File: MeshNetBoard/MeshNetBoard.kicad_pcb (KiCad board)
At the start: 2 copper layers, 35 x 21 mm, 9 parts, among them J1 Conn_01x02, U1 XIAO-ESP32-S3-DIP, U2 TPS631000DRLR

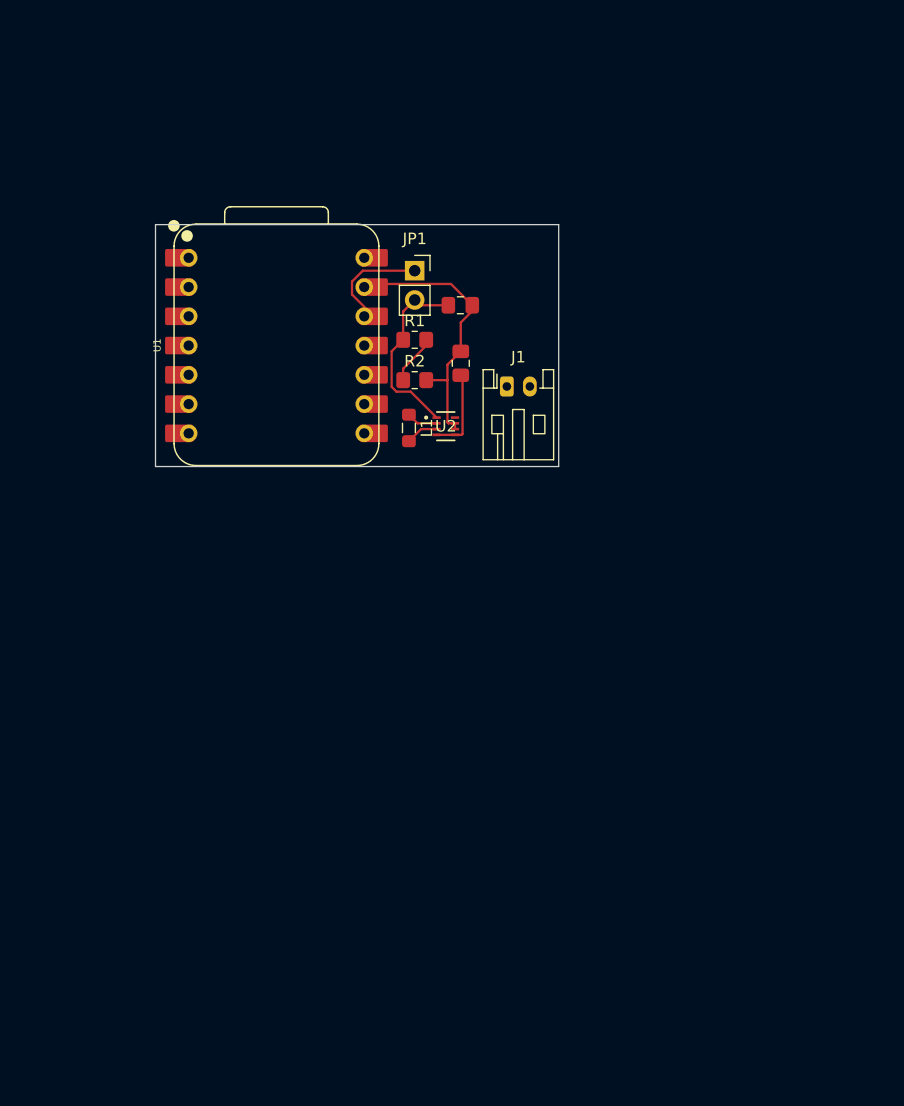
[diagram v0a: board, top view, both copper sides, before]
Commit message: for pdr
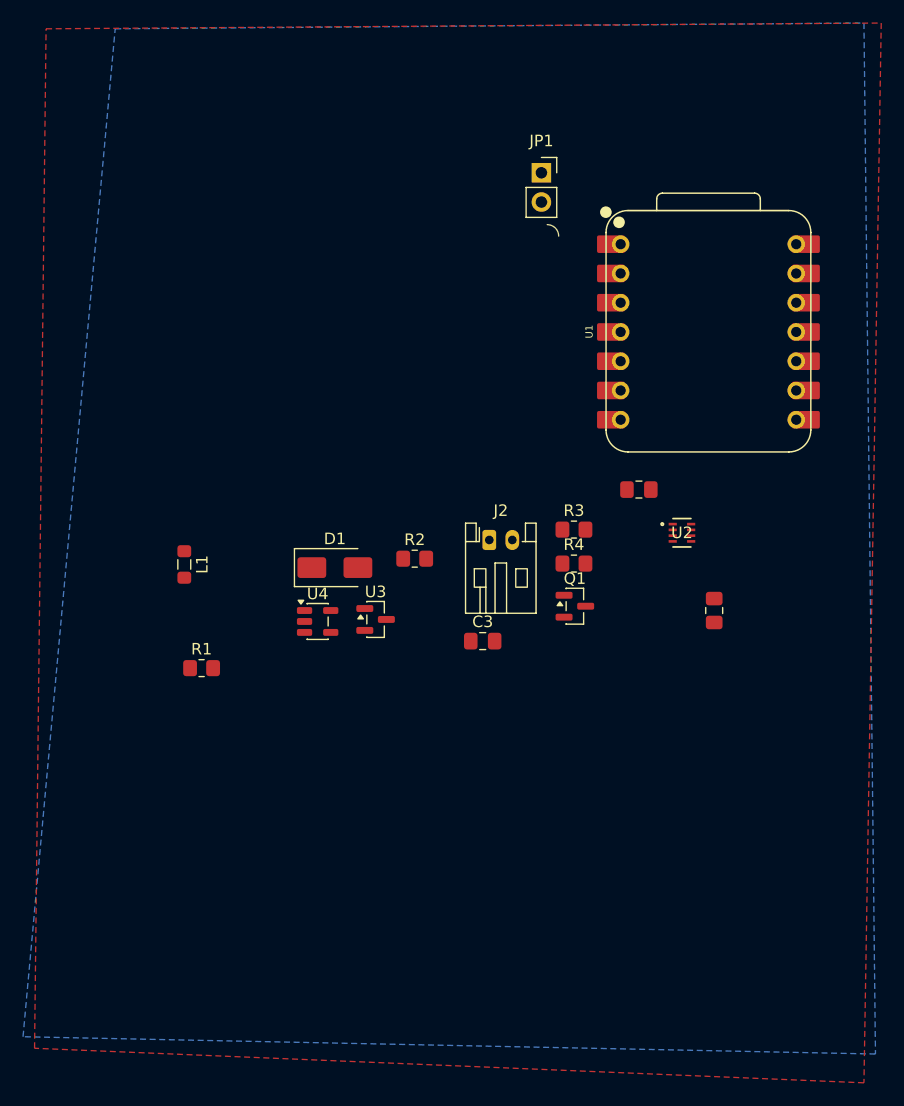
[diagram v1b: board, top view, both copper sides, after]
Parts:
- removed J1: Conn_01x02, Connector_JST:JST_PH_S2B-PH-K_1x02_P2.00mm_Horizontal
- added C3: 0.1μF, Capacitor_SMD:C_0805_2012Metric_Pad1.18x1.45mm_HandSolder, F.Cu at (88.4, 75.2)
- added D1: SS14, Diode_SMD:D_SMA, F.Cu at (75.6, 68.8)
- added J2: Conn_01x02, Connector_JST:JST_PH_S2B-PH-K_1x02_P2.00mm_Horizontal, F.Cu at (89.0, 66.4)
- added Q1: Q_PMOS_GSD, Package_TO_SOT_SMD:SOT-23, F.Cu at (96.4, 72.1)
- added R3: 510k, Resistor_SMD:R_0805_2012Metric_Pad1.20x1.40mm_HandSolder, F.Cu at (96.3, 65.5)
- added R4: 1M, Resistor_SMD:R_0805_2012Metric_Pad1.20x1.40mm_HandSolder, F.Cu at (96.3, 68.4)
- added U3: LM4040DBZ-2.0, Package_TO_SOT_SMD:SOT-23, F.Cu at (79.1, 73.3)
- added U4: MAX9031AU, Package_TO_SOT_SMD:SOT-23-5, F.Cu at (74.1, 73.5)
- moved U1 37.5 mm to (108.0, 48.3)
- moved R1 34.0 mm to (64.0, 77.5)
- moved C2 30.7 mm to (108.5, 72.5)
- moved L1 22.8 mm to (62.5, 68.5)
- moved U2 22.5 mm to (105.7, 65.8)
- moved C1 22.3 mm to (102.0, 62.0)
- moved R2 15.5 mm to (82.5, 68.0)
- moved JP1 13.9 mm to (93.5, 34.5)
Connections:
- C2 pad 1: +BATT -> Net-(Q1-S)
- JP1 pad 1: Net-(JP1-A) -> Net-(D1-A)
- U1 pad 12: Net-(JP1-A) -> Net-(D1-K)
- U2 pad 4: +BATT -> Net-(Q1-S)
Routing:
- net GND: track 23.5 -> 0.00 mm
- net Net-(JP1-B): track 16.5 -> 0.00 mm
- net Net-(JP1-A): track 9.64 -> 0.00 mm
- net +BATT: track 7.45 -> 0.00 mm
- net Net-(U2-FB): track 4.33 -> 0.00 mm
- net Net-(U2-LX1): track 2.83 -> 0.00 mm
- net Net-(U2-LX2): track 2.71 -> 0.00 mm
- added copper zone on B.Cu, net +BATT
- added copper zone on F.Cu, net GND
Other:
- board size 35 x 21 mm -> 1 x 1 mm
